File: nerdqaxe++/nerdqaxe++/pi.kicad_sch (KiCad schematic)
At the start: 20 parts, among them J5 Conn_01x12-Socket, J6 Conn_01x12-Socket, J7 Conn_01x12-Header, J8 Conn_01x12-Header, M1 Fan_4pin, M2 Fan_4pin, U30 T-Display-S3, U32 EMC2302-1, U33 TXU0102-DCU, U37 TMP1075, U38 TMP1075

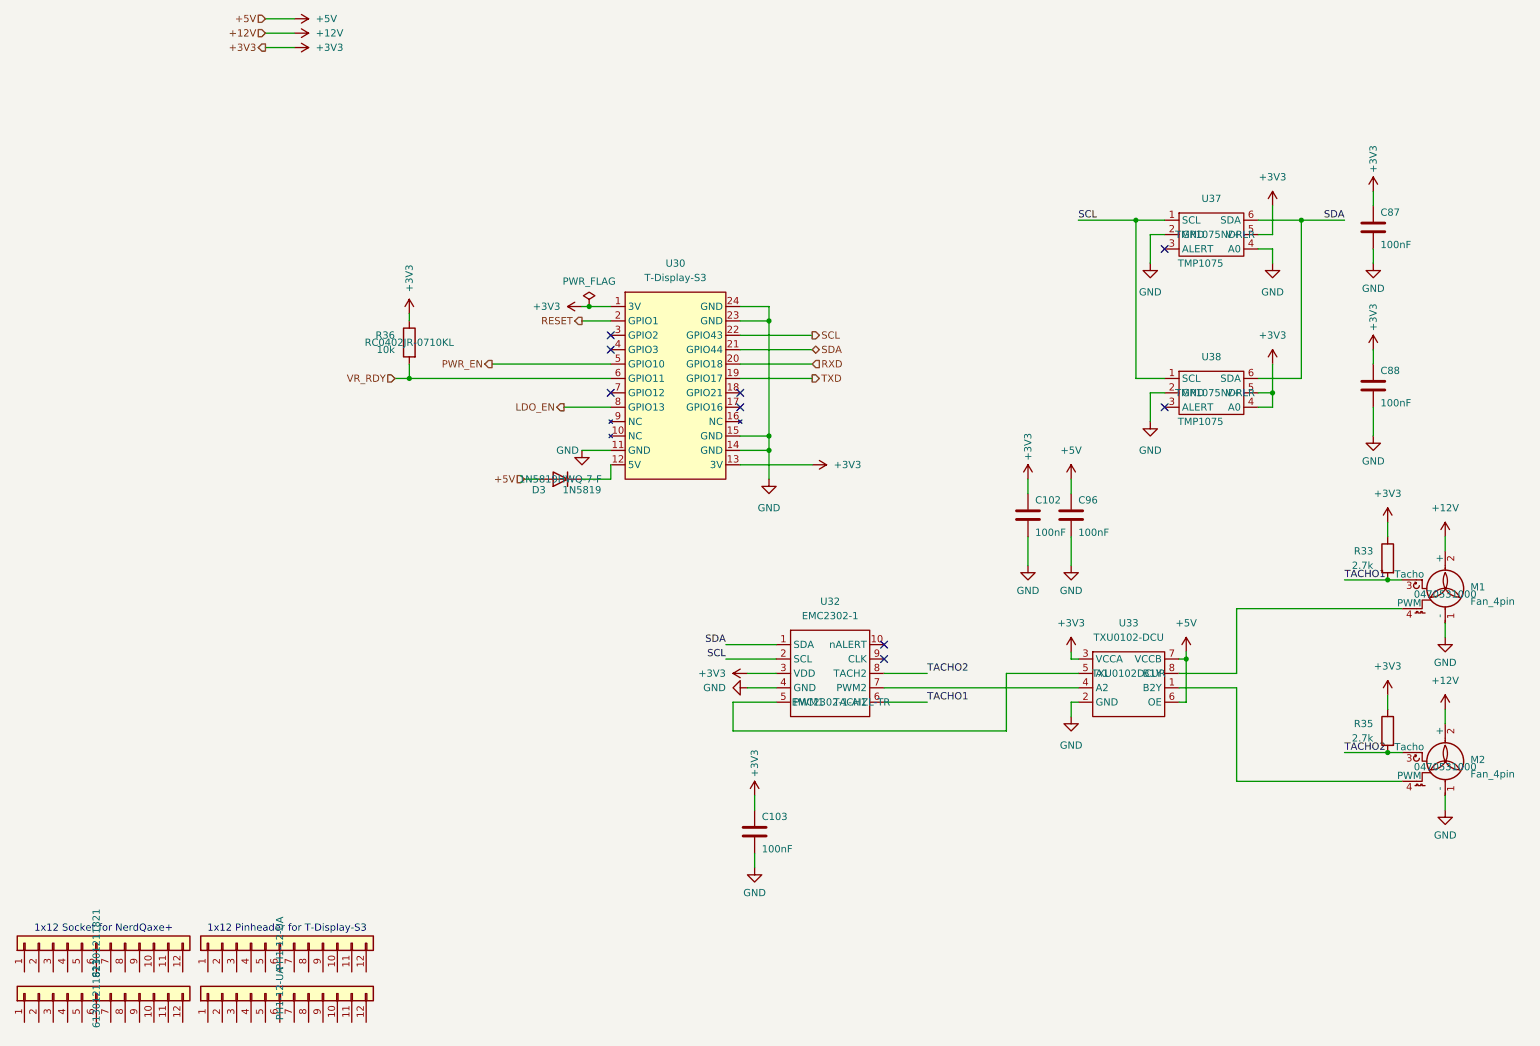
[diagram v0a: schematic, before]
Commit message: finishing up
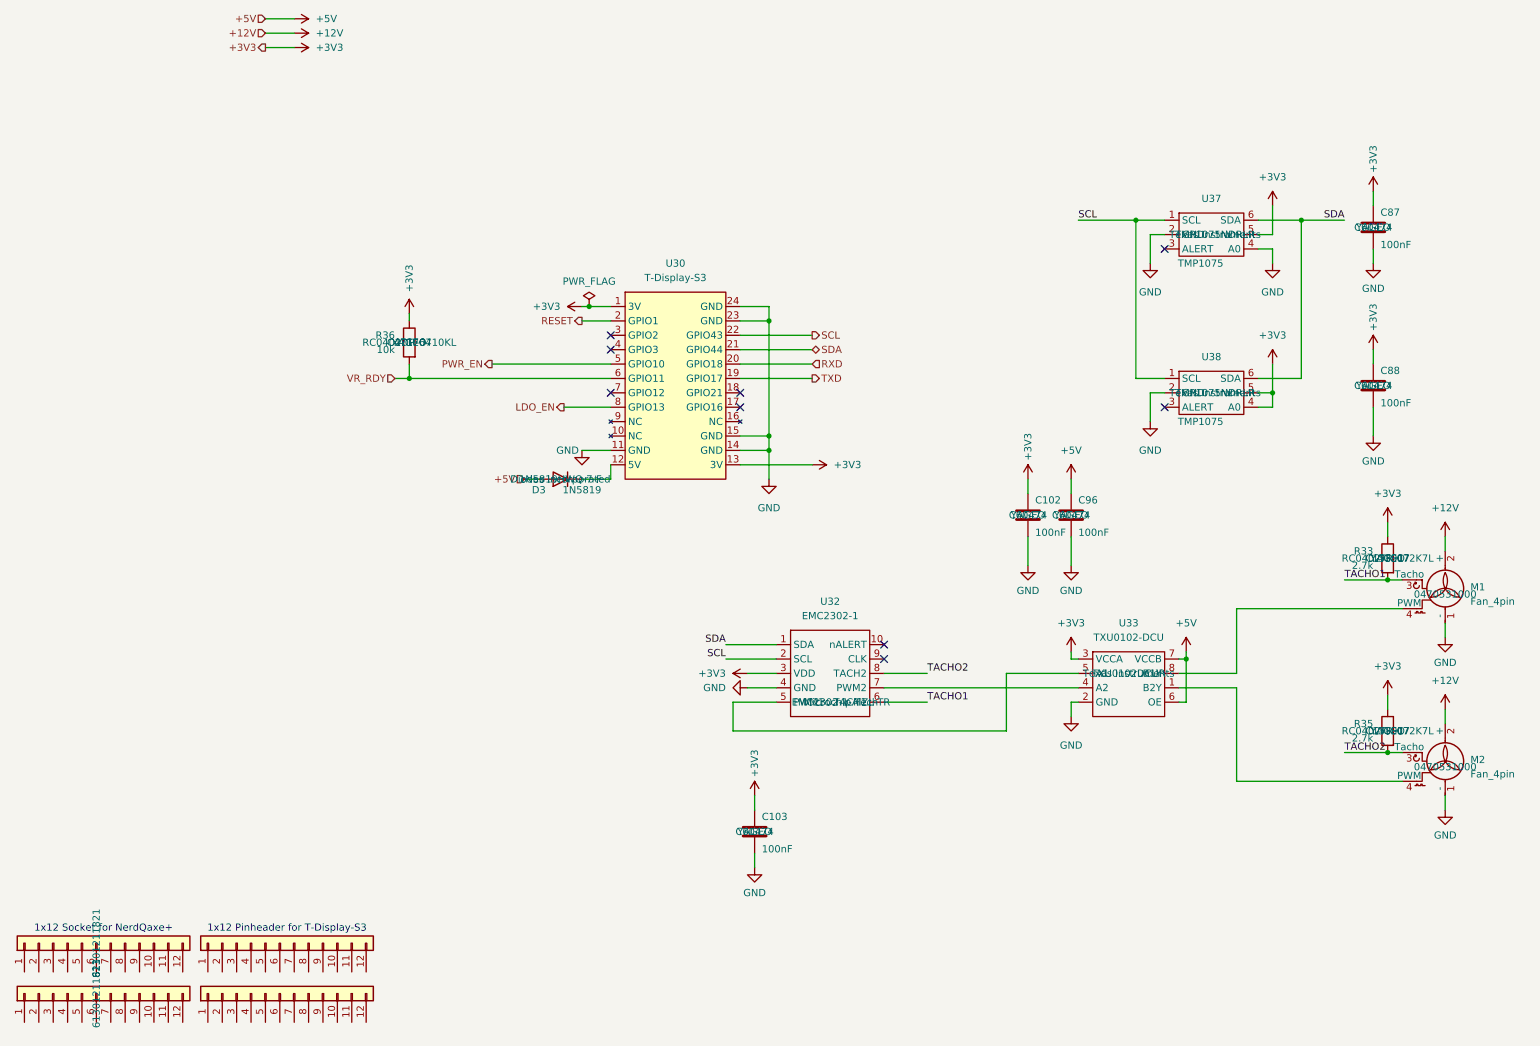
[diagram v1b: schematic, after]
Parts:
- C102, C103, C87, C88, C96: LCSC (none) -> C60474; Manufacturer  (none) -> YAGEO; PARTNO CL05A104KO5NNNC -> CC0402KRX7R7BB104
- D3: Manufacturer  (none) -> Diodes Incorporated
- J7, J8: PARTNO PH1-12-UA -> (none)
- R33, R35: LCSC (none) -> C138017; Manufacturer  (none) -> YAGEO; PARTNO (none) -> RC0402FR-072K7L
- R36: LCSC (none) -> C471764; Manufacturer  (none) -> YAGEO; PARTNO RC0402JR-0710KL -> RC0402DR-0710KL
- U32: Manufacturer  (none) -> Microchip Tech
- U33, U37, U38: Manufacturer  (none) -> Texas Instruments
